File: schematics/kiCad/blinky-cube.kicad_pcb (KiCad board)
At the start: 2 copper layers, 86.6 x 49.7 mm, 26 parts, among them J1 Screw_Terminal_01x03, J2 Screw_Terminal_01x03, J3 Screw_Terminal_01x03, J4 Screw_Terminal_01x03, SW1 SW_Push, U1 Pico, U2 LM4040LP-3, U3 BZX84C3V3, U4 BZX84C3V3, U5 BZX84C3V3

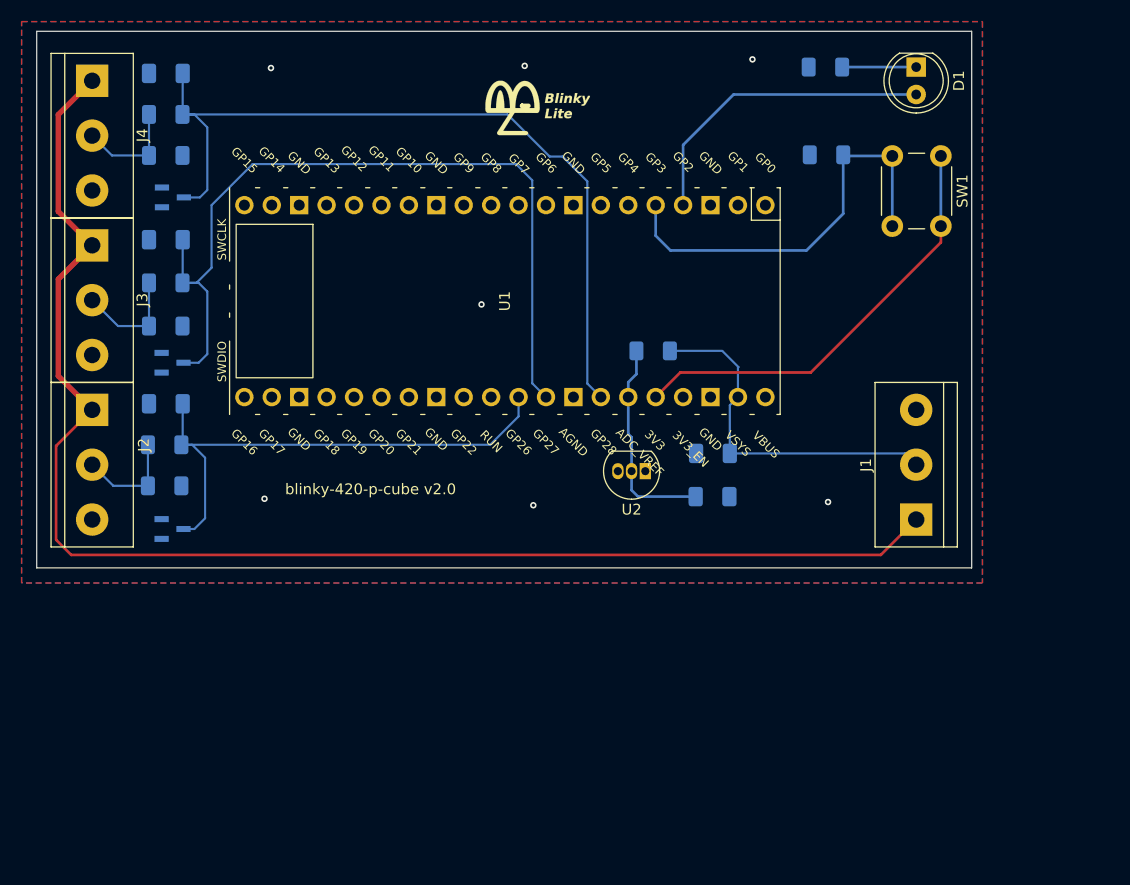
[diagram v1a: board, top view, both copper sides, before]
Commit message: layout complete
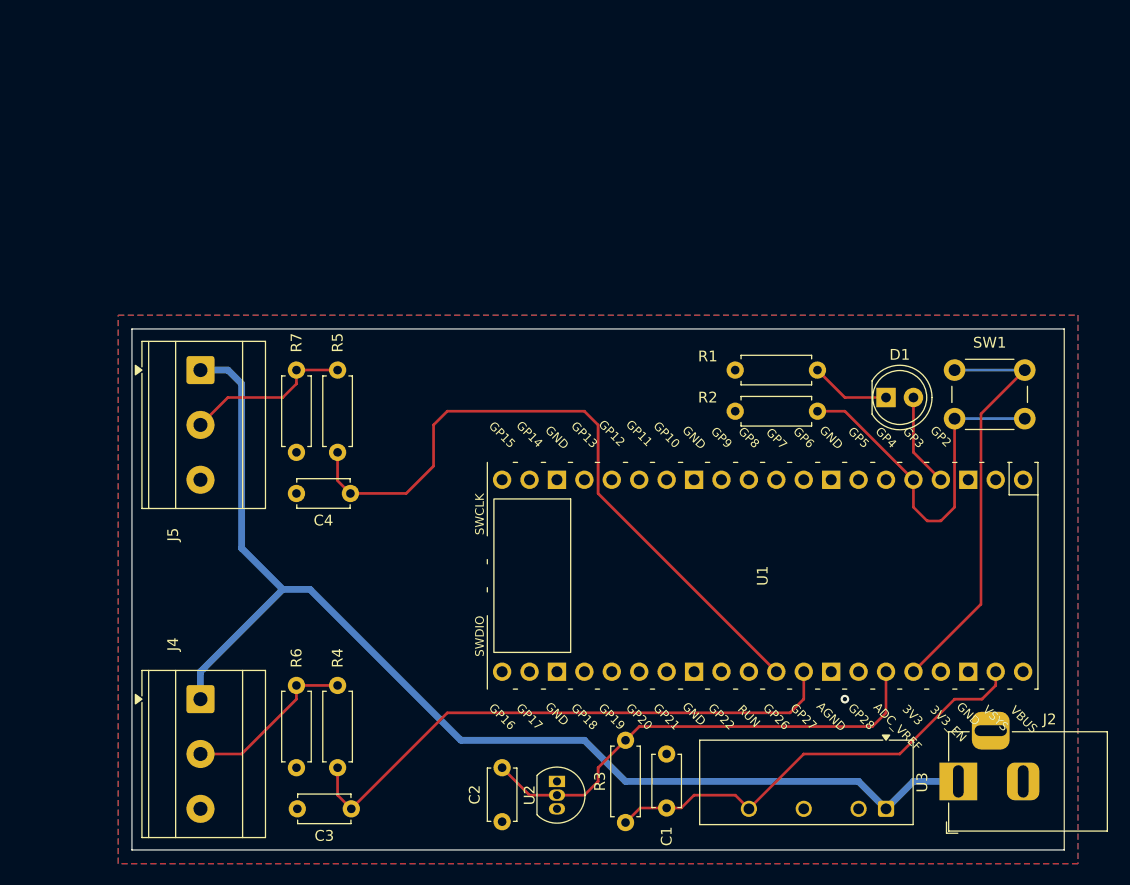
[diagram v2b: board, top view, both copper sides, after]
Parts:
- removed C6: 1uF, Capacitor_SMD:C_1206_3216Metric_Pad1.33x1.80mm_HandSolder
- removed G***: LOGO, blinkyLiteLogo:blinkyLiteLogo
- removed J1, J3: Screw_Terminal_01x03, TerminalBlock:TerminalBlock_bornier-3_P5.08mm
- removed R8, R9: 100, Resistor_SMD:R_1206_3216Metric_Pad1.30x1.75mm_HandSolder
- removed U4, U5: BZX84C3V3, BZX84C3V3:SOT91P240X110-3N
- added J5: Screw_Terminal_01x03, TerminalBlock_Phoenix:TerminalBlock_Phoenix_MKDS-3-3-5.08_1x03_P5.08mm_Horizontal, F.Cu at (115.6, 81.3)
- C1, C2, C3, C4: footprint Capacitor_SMD:C_1206_3216Metric_Pad1.33x1.80mm_HandSolder -> Capacitor_THT:C_Disc_D4.7mm_W2.5mm_P5.00mm; moved to F.Cu
- J2: value Screw_Terminal_01x03 -> Barrel_Jack_Switch; footprint TerminalBlock:TerminalBlock_bornier-3_P5.08mm -> Connector_BarrelJack:BarrelJack_Horizontal
- J4: footprint TerminalBlock:TerminalBlock_bornier-3_P5.08mm -> TerminalBlock_Phoenix:TerminalBlock_Phoenix_MKDS-3-3-5.08_1x03_P5.08mm_Horizontal
- R1, R2, R3: footprint Resistor_SMD:R_1206_3216Metric_Pad1.30x1.75mm_HandSolder -> Resistor_THT:R_Axial_DIN0207_L6.3mm_D2.5mm_P7.62mm_Horizontal; moved to F.Cu
- R4, R5, R6, R7: value 100 -> 120; footprint Resistor_SMD:R_1206_3216Metric_Pad1.30x1.75mm_HandSolder -> Resistor_THT:R_Axial_DIN0207_L6.3mm_D2.5mm_P7.62mm_Horizontal; moved to F.Cu
- U3: value BZX84C3V3 -> TBA2-2411; footprint BZX84C3V3:SOT91P240X110-3N -> Converter_DCDC:Converter_DCDC_TRACO_TBA2-xxxx_Single_THT; moved to F.Cu
- moved J2 87.3 mm to (185.8, 119.4), turned to 180 degrees
- moved U3 71.0 mm to (179.1, 121.9), turned to -90 degrees
- moved J4 58.1 mm to (115.6, 111.8)
- moved C3 55.4 mm to (129.5, 121.9)
- moved C2 45.9 mm to (143.5, 118.1), turned to -90 degrees
- moved R3 43.8 mm to (154.9, 123.2), turned to 90 degrees
- moved C4 42.5 mm to (129.5, 92.7)
- moved R6 35.4 mm to (124.5, 110.5), turned to -90 degrees
- moved U1 34.9 mm to (167.6, 100.3)
- moved C1 33.1 mm to (158.8, 121.8), turned to 90 degrees
- moved D1 30.7 mm to (179.1, 83.8), turned to 0 degrees
- moved U2 29.9 mm to (148.6, 119.4), turned to -90 degrees
- moved R1 29.3 mm to (165.1, 81.3)
- moved R4 24.5 mm to (128.3, 110.5), turned to -90 degrees
- moved R2 23.8 mm to (172.7, 85.1)
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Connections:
- C1 pad 1: Net-(J1-Pin_2) -> Net-(U1-VSYS)
- C2 pad 1: /P31 -> Net-(U1-ADC_VREF)
- C3 pad 1: /P32 -> Net-(U1-GPIO27_ADC1)
- C4 pad 1: /P34 -> Net-(U1-GPIO26_ADC0)
- J2 pad 1: /Vext -> Net-(J4-Pin_1)
- J2 pad 2: Net-(J2-Pin_2) -> GND
- J2 pad 3: GND -> unconnected-(J2-Pad3)
- J4 pad 1: /Vext -> Net-(J4-Pin_1)
- R3 pad 1: Net-(J1-Pin_2) -> Net-(U1-VSYS)
- R4 pad 1: GND -> Net-(J4-Pin_2)
- R4 pad 2: Net-(J2-Pin_2) -> Net-(U1-GPIO27_ADC1)
- R5 pad 1: /P31 -> Net-(J5-Pin_2)
- R5 pad 2: Net-(J2-Pin_2) -> Net-(U1-GPIO26_ADC0)
- R6 pad 1: GND -> Net-(J4-Pin_2)
- R6 pad 2: Net-(J3-Pin_2) -> GND
- R7 pad 1: /P32 -> Net-(J5-Pin_2)
- R7 pad 2: Net-(J3-Pin_2) -> GND
- U1 pad 31: /P31 -> Net-(U1-GPIO26_ADC0)
- U1 pad 32: /P32 -> Net-(U1-GPIO27_ADC1)
- U1 pad 34: /P34 -> unconnected-(U1-GPIO28_ADC2-Pad34)
- U1 pad 39: Net-(J1-Pin_2) -> Net-(U1-VSYS)
- U3 pad 1: GND -> Net-(J4-Pin_1)
- U3 pad 2: unconnected-(U3-NC-Pad2) -> GND
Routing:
- net /Vext: track 131.1 -> 0.00 mm
- net Net-(J4-Pin_1): track 0.00 -> 110.3 mm
- net /P32: track 76.6 -> 0.00 mm
- net /P34: track 75.4 -> 0.00 mm
- net Net-(U1-GPIO26_ADC0): track 0.00 -> 62.9 mm
- net Net-(U1-GPIO27_ADC1): track 0.00 -> 53.0 mm
- net /P31: track 48.7 -> 0.00 mm
- net Net-(U1-VSYS): track 0.00 -> 41.9 mm
- net Net-(J1-Pin_2): track 33.0 -> 0.00 mm
- net Net-(U1-ADC_VREF): track 19.5 -> 44.3 mm
- net Net-(D1-A): track 29.1 -> 8.67 mm
- net Net-(J5-Pin_2): track 0.00 -> 15.5 mm
- net Net-(J3-Pin_2): track 10.3 -> 0.00 mm
- net Net-(J2-Pin_2): track 9.77 -> 0.00 mm
- net Net-(J4-Pin_2): track 9.82 -> 16.1 mm
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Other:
- board size 86.6 x 49.7 mm -> 86.4 x 48.3 mm
- board text removed: "blinky-420-p-cube v2.0"
